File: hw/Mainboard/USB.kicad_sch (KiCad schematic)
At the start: 8 parts, among them J25 USB2.0_HOST_TYPE_C

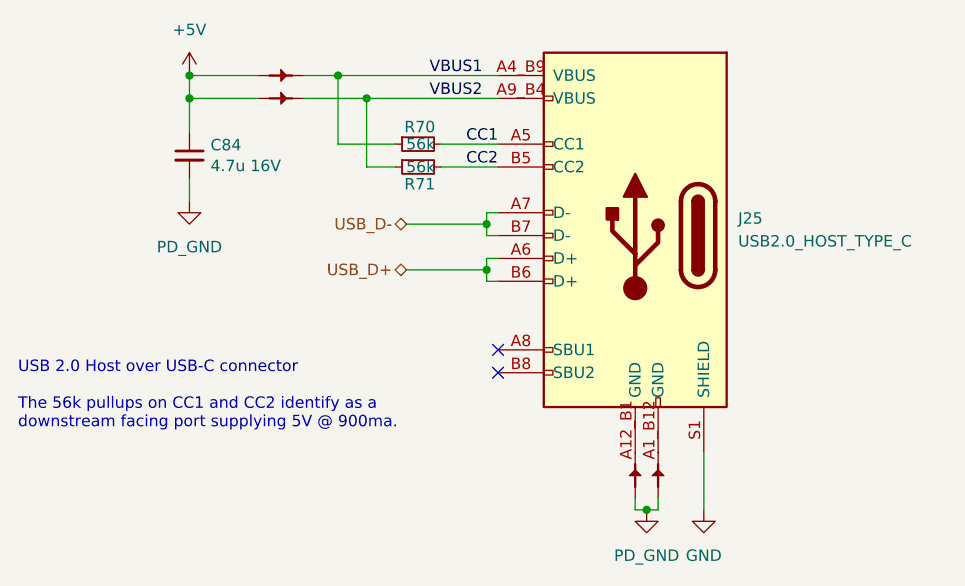
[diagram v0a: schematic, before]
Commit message: hw: 25x2 header (wip)
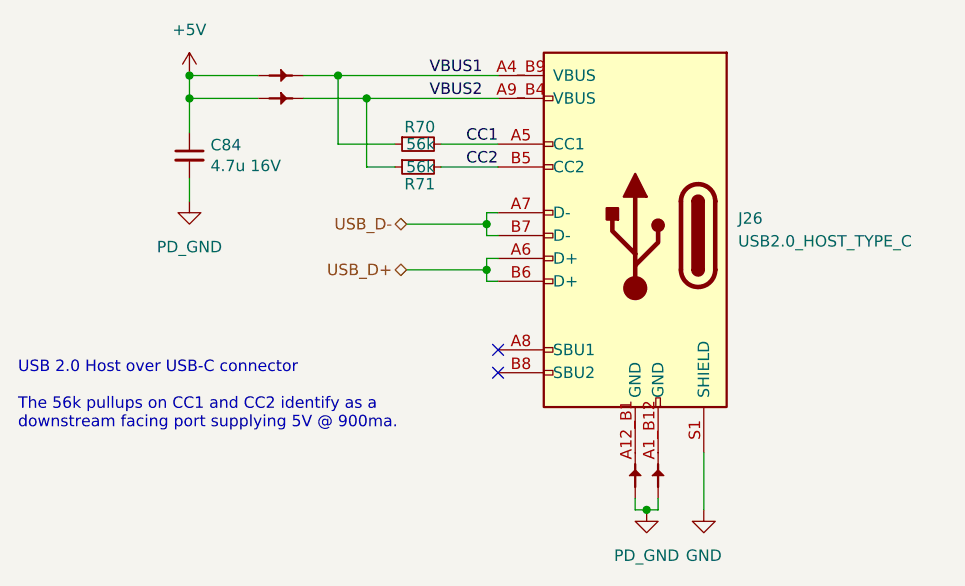
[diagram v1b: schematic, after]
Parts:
- renumbered J25 to J26
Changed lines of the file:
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@@
   (symbol (lib_id "PET:PD_GND") (at 102.87 88.9 0) (unit 1)
     (in_bom yes) (on_board yes) (fields_autoplaced)
-    (property "Reference" "#PWR0150" (id 0) (at 102.87 95.25 0)
+    (property "Reference" "#PWR0152" (id 0) (at 102.87 95.25 0)
       (effects (font (size 1.27 1.27)) hide)
     )
@@
   (symbol (lib_id "JLCPCB:USB_C_Receptacle_USB2.0") (at 152.4 92.71 0) (mirror y) (unit 1)
     (in_bom yes) (on_board yes) (fields_autoplaced)
-    (property "Reference" "J25" (id 0) (at 163.83 90.8049 0)
+    (property "Reference" "J26" (id 0) (at 163.83 90.8049 0)
       (effects (font (size 1.27 1.27)) (justify right))
     )
@@
   (symbol (lib_id "power:+5V") (at 102.87 74.93 0) (mirror y) (unit 1)
     (in_bom yes) (on_board yes) (fields_autoplaced)
-    (property "Reference" "#PWR0149" (id 0) (at 102.87 78.74 0)
+    (property "Reference" "#PWR0151" (id 0) (at 102.87 78.74 0)
       (effects (font (size 1.27 1.27)) hide)
     )
@@
   (symbol (lib_id "PET:PD_GND") (at 153.67 123.19 0) (unit 1)
     (in_bom yes) (on_board yes) (fields_autoplaced)
-    (property "Reference" "#PWR0151" (id 0) (at 153.67 129.54 0)
+    (property "Reference" "#PWR0153" (id 0) (at 153.67 129.54 0)
       (effects (font (size 1.27 1.27)) hide)
     )
@@
   (symbol (lib_id "power:GND") (at 160.02 123.19 0) (unit 1)
     (in_bom yes) (on_board yes) (fields_autoplaced)
-    (property "Reference" "#PWR0152" (id 0) (at 160.02 129.54 0)
+    (property "Reference" "#PWR0154" (id 0) (at 160.02 129.54 0)
       (effects (font (size 1.27 1.27)) hide)
     )

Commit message: hw: 2x config switch (wip)
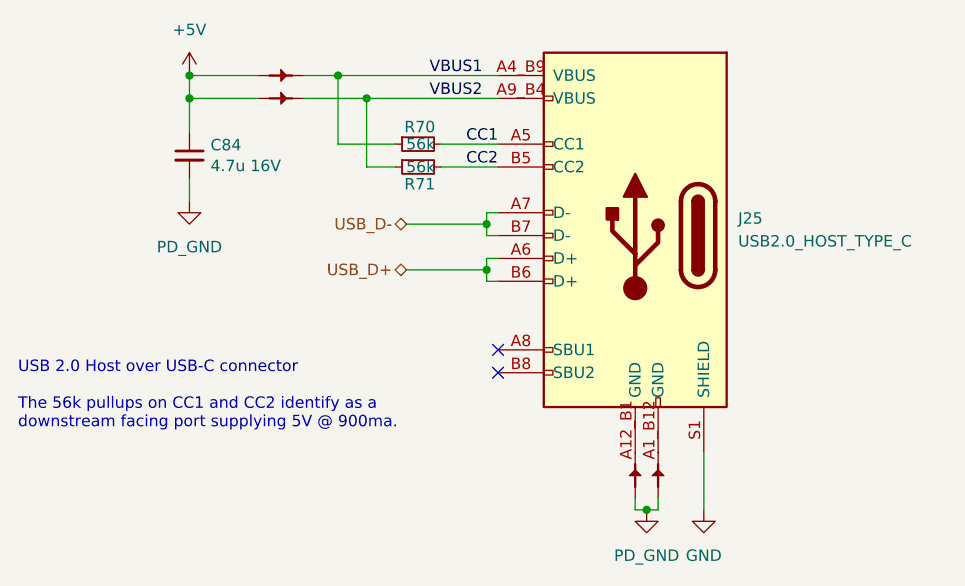
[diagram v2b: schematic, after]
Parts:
- renumbered J26 to J25
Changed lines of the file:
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@@
   (symbol (lib_id "PET:PD_GND") (at 102.87 88.9 0) (unit 1)
     (in_bom yes) (on_board yes) (fields_autoplaced)
-    (property "Reference" "#PWR0152" (id 0) (at 102.87 95.25 0)
+    (property "Reference" "#PWR0158" (id 0) (at 102.87 95.25 0)
       (effects (font (size 1.27 1.27)) hide)
     )
@@
   (symbol (lib_id "JLCPCB:USB_C_Receptacle_USB2.0") (at 152.4 92.71 0) (mirror y) (unit 1)
     (in_bom yes) (on_board yes) (fields_autoplaced)
-    (property "Reference" "J26" (id 0) (at 163.83 90.8049 0)
+    (property "Reference" "J25" (id 0) (at 163.83 90.8049 0)
       (effects (font (size 1.27 1.27)) (justify right))
     )
@@
   (symbol (lib_id "power:+5V") (at 102.87 74.93 0) (mirror y) (unit 1)
     (in_bom yes) (on_board yes) (fields_autoplaced)
-    (property "Reference" "#PWR0151" (id 0) (at 102.87 78.74 0)
+    (property "Reference" "#PWR0157" (id 0) (at 102.87 78.74 0)
       (effects (font (size 1.27 1.27)) hide)
     )
@@
   (symbol (lib_id "PET:PD_GND") (at 153.67 123.19 0) (unit 1)
     (in_bom yes) (on_board yes) (fields_autoplaced)
-    (property "Reference" "#PWR0153" (id 0) (at 153.67 129.54 0)
+    (property "Reference" "#PWR0159" (id 0) (at 153.67 129.54 0)
       (effects (font (size 1.27 1.27)) hide)
     )
@@
   (symbol (lib_id "power:GND") (at 160.02 123.19 0) (unit 1)
     (in_bom yes) (on_board yes) (fields_autoplaced)
-    (property "Reference" "#PWR0154" (id 0) (at 160.02 129.54 0)
+    (property "Reference" "#PWR0160" (id 0) (at 160.02 129.54 0)
       (effects (font (size 1.27 1.27)) hide)
     )
